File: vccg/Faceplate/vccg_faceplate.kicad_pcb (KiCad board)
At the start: 2 copper layers, 50.8 x 128.5 mm, 19 parts

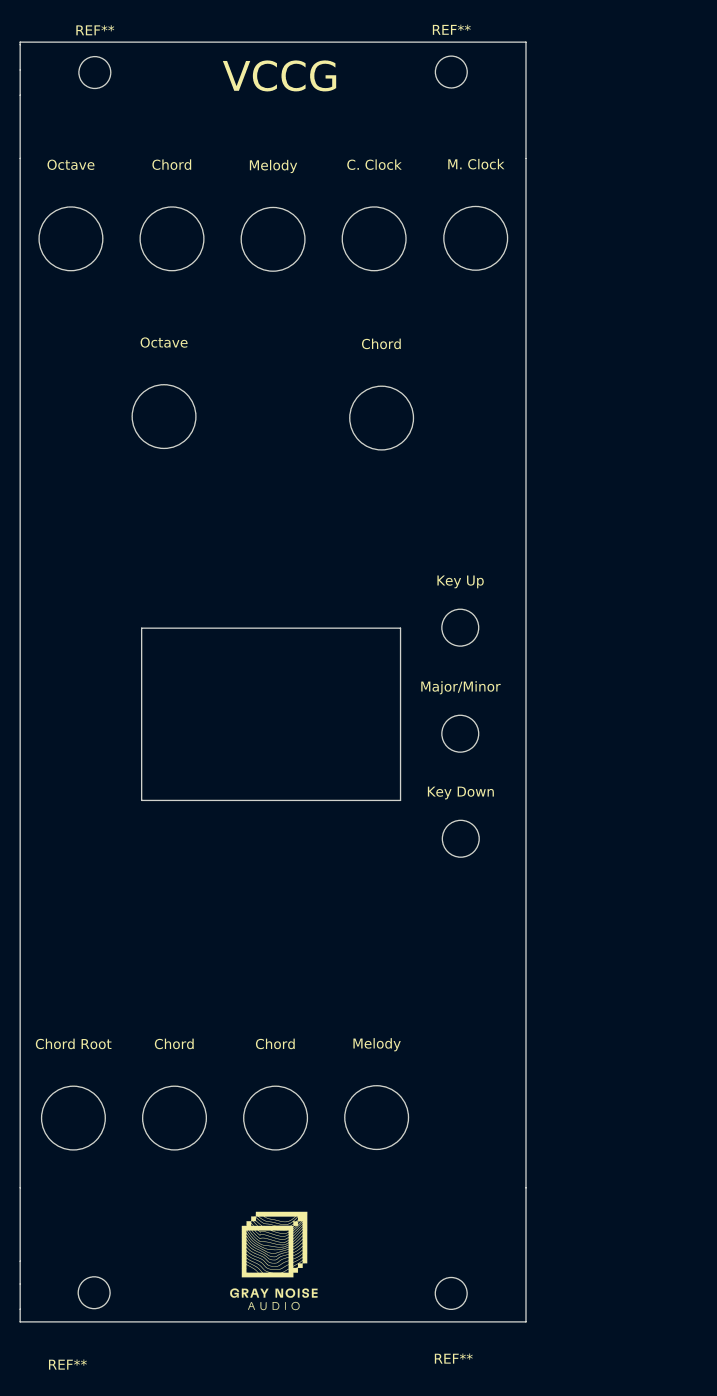
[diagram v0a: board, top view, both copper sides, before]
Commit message: Adding Molly's shiny new faceplate design
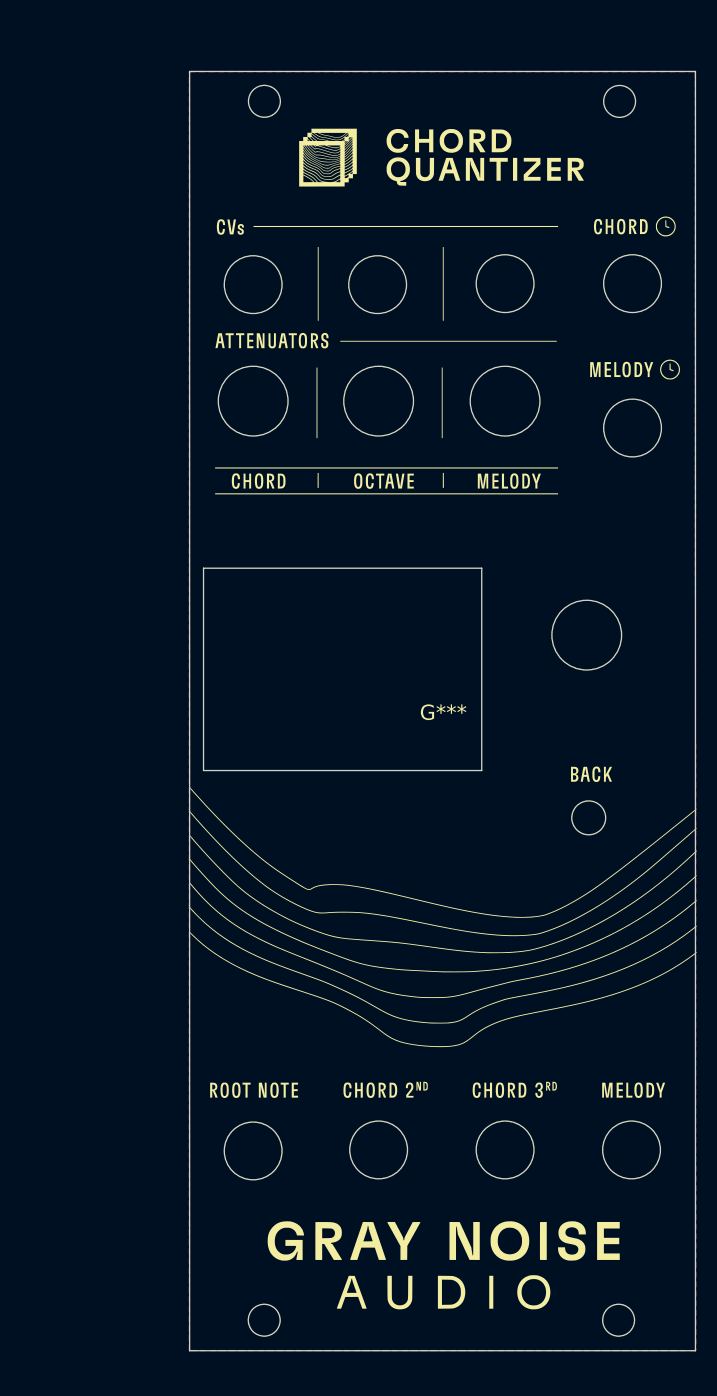
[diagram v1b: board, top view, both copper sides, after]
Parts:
- removed C. Clock: MountingHole_6.4mm_M6, MountingHole:MountingHole_6.4mm_M6
- removed Chord (x4), Melody (x2), Octave (x2): MountingHole_6.4mm_M6, MountingHole:MountingHole_6.4mm_M6
- removed Chord Root: MountingHole_6.4mm_M6, MountingHole:MountingHole_6.4mm_M6
- removed the G*** at (203.3, 134.9)
- removed Key Down: MountingHole_3.7mm, MountingHole:MountingHole_3.7mm
- removed Key Up: MountingHole_3.7mm, MountingHole:MountingHole_3.7mm
- removed M. Clock: MountingHole_6.4mm_M6, MountingHole:MountingHole_6.4mm_M6
- removed Major/Minor: MountingHole_3.7mm, MountingHole:MountingHole_3.7mm
- removed REF** (x4): MountingHole_3.2mm_M3, MountingHole:MountingHole_3.2mm_M3
- added G***: LOGO, SynthStuff:vccg_faceplate, F.Cu at (220.3, 79.8)
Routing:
- added copper zone on F.Cu, net (none)
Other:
- outline, holes or cut-outs redrawn
- net class Default removed
- board text added: "Back button"
- board text added: "Chord 2nd"
- board text added: "Chord 3rd"
- board text added: "Chord CV"
- board text added: "Chord Clock"
- board text added: "Chord attenuator"
- board text added: "Melody"
- board text added: "Melody Attenuator"
- board text added: "Melody CV"
- board text added: "Melody Clock"
- board text added: "Octave Attenuator"
- board text added: "Octave CV"
- board text added: "Root note"
- board text added: "Screen"
- board text added: "Selection Dial"
- board text removed: "VCCG"
